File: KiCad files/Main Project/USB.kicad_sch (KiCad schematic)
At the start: 4 parts, among them J2 USB_C_Receptacle_USB2.0

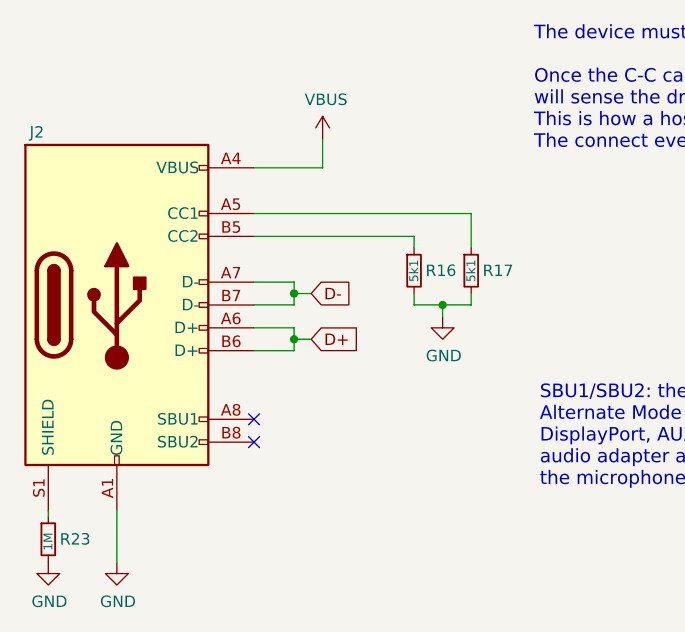
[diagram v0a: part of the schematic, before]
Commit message: shematic update
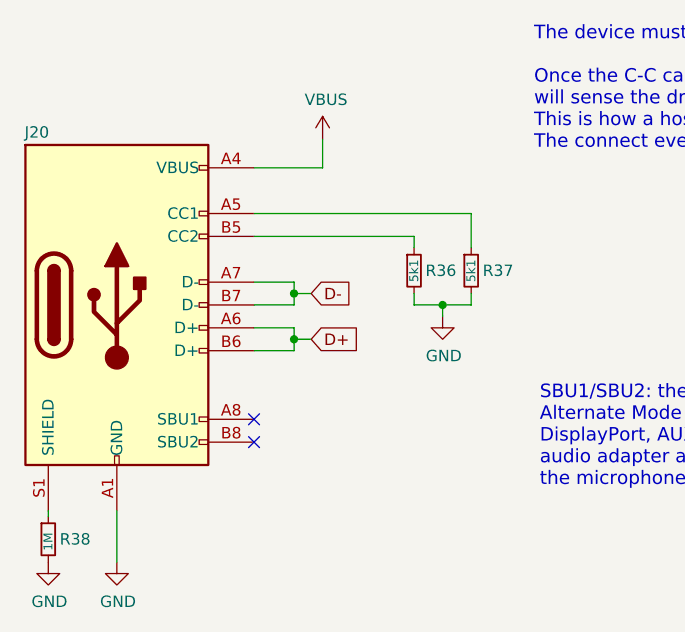
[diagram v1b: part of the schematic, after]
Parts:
- renumbered J2 to J20, R16 to R36, R17 to R37, R23 to R38
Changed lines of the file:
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@@
   (symbol (lib_id "Connector:USB_C_Receptacle_USB2.0") (at 96.52 94.615 0) (unit 1)
     (in_bom yes) (on_board yes)
-    (property "Reference" "J2" (id 0) (at 87.63 75.438 0))
+    (property "Reference" "J20" (id 0) (at 87.63 75.438 0))
     (property "Value" "USB_C_Receptacle_USB2.0" (id 1) (at 99.2378 74.9046 0)
       (effects (font (size 1.27 1.27)) hide)
@@
   (symbol (lib_id "power:VBUS") (at 119.38 76.2 0) (unit 1)
     (in_bom yes) (on_board yes)
-    (property "Reference" "#PWR070" (id 0) (at 119.38 80.01 0)
+    (property "Reference" "#PWR077" (id 0) (at 119.38 80.01 0)
       (effects (font (size 1.27 1.27)) hide)
     )
@@
   (symbol (lib_id "power:GND") (at 96.52 123.19 0) (unit 1)
     (in_bom yes) (on_board yes)
-    (property "Reference" "#PWR069" (id 0) (at 96.52 129.54 0)
+    (property "Reference" "#PWR080" (id 0) (at 96.52 129.54 0)
       (effects (font (size 1.27 1.27)) hide)
     )
@@
   (symbol (lib_id "Device:R_Small") (at 129.54 90.805 0) (unit 1)
     (in_bom yes) (on_board yes)
-    (property "Reference" "R16" (id 0) (at 130.81 90.805 0)
+    (property "Reference" "R36" (id 0) (at 130.81 90.805 0)
       (effects (font (size 1.27 1.27)) (justify left))
     )
@@
   (symbol (lib_id "Device:R_Small") (at 135.89 90.805 0) (unit 1)
     (in_bom yes) (on_board yes)
-    (property "Reference" "R17" (id 0) (at 137.16 90.805 0)
+    (property "Reference" "R37" (id 0) (at 137.16 90.805 0)
       (effects (font (size 1.27 1.27)) (justify left))
     )
@@
   (symbol (lib_id "power:GND") (at 132.715 95.885 0) (unit 1)
     (in_bom yes) (on_board yes)
-    (property "Reference" "#PWR072" (id 0) (at 132.715 102.235 0)
+    (property "Reference" "#PWR078" (id 0) (at 132.715 102.235 0)
       (effects (font (size 1.27 1.27)) hide)
     )
@@
   (symbol (lib_id "Device:R_Small") (at 88.9 120.65 0) (unit 1)
     (in_bom yes) (on_board yes)
-    (property "Reference" "R23" (id 0) (at 90.17 120.65 0)
+    (property "Reference" "R38" (id 0) (at 90.17 120.65 0)
       (effects (font (size 1.27 1.27)) (justify left))
     )
@@
   (symbol (lib_id "power:GND") (at 88.9 123.19 0) (unit 1)
     (in_bom yes) (on_board yes)
-    (property "Reference" "#PWR0272" (id 0) (at 88.9 129.54 0)
+    (property "Reference" "#PWR079" (id 0) (at 88.9 129.54 0)
       (effects (font (size 1.27 1.27)) hide)
     )

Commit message: update
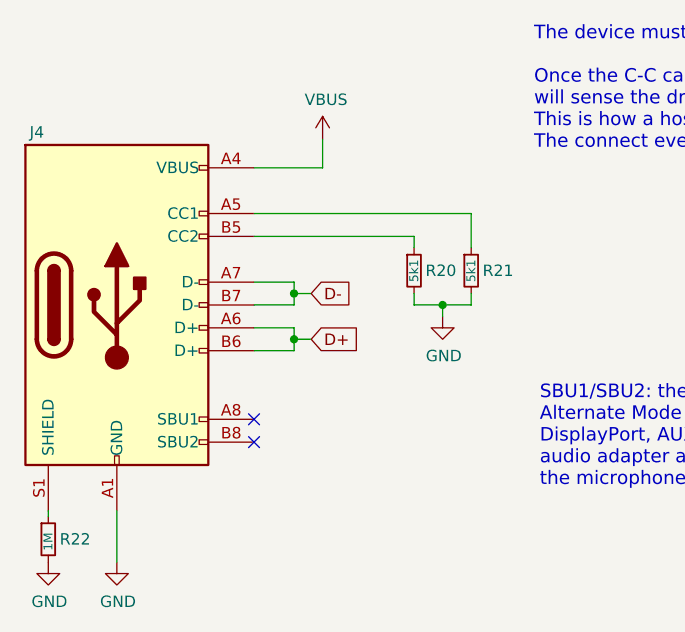
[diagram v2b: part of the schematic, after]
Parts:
- renumbered J20 to J4, R36 to R20, R37 to R21, R38 to R22
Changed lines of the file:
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@@
   (symbol (lib_id "Connector:USB_C_Receptacle_USB2.0") (at 96.52 94.615 0) (unit 1)
     (in_bom yes) (on_board yes)
-    (property "Reference" "J20" (id 0) (at 87.63 75.438 0))
+    (property "Reference" "J4" (id 0) (at 87.63 75.438 0))
     (property "Value" "USB_C_Receptacle_USB2.0" (id 1) (at 99.2378 74.9046 0)
       (effects (font (size 1.27 1.27)) hide)
@@
   (symbol (lib_id "power:VBUS") (at 119.38 76.2 0) (unit 1)
     (in_bom yes) (on_board yes)
-    (property "Reference" "#PWR077" (id 0) (at 119.38 80.01 0)
+    (property "Reference" "#PWR061" (id 0) (at 119.38 80.01 0)
       (effects (font (size 1.27 1.27)) hide)
     )
@@
   (symbol (lib_id "power:GND") (at 96.52 123.19 0) (unit 1)
     (in_bom yes) (on_board yes)
-    (property "Reference" "#PWR080" (id 0) (at 96.52 129.54 0)
+    (property "Reference" "#PWR064" (id 0) (at 96.52 129.54 0)
       (effects (font (size 1.27 1.27)) hide)
     )
@@
   (symbol (lib_id "Device:R_Small") (at 129.54 90.805 0) (unit 1)
     (in_bom yes) (on_board yes)
-    (property "Reference" "R36" (id 0) (at 130.81 90.805 0)
+    (property "Reference" "R20" (id 0) (at 130.81 90.805 0)
       (effects (font (size 1.27 1.27)) (justify left))
     )
@@
   (symbol (lib_id "Device:R_Small") (at 135.89 90.805 0) (unit 1)
     (in_bom yes) (on_board yes)
-    (property "Reference" "R37" (id 0) (at 137.16 90.805 0)
+    (property "Reference" "R21" (id 0) (at 137.16 90.805 0)
       (effects (font (size 1.27 1.27)) (justify left))
     )
@@
   (symbol (lib_id "power:GND") (at 132.715 95.885 0) (unit 1)
     (in_bom yes) (on_board yes)
-    (property "Reference" "#PWR078" (id 0) (at 132.715 102.235 0)
+    (property "Reference" "#PWR062" (id 0) (at 132.715 102.235 0)
       (effects (font (size 1.27 1.27)) hide)
     )
@@
   (symbol (lib_id "Device:R_Small") (at 88.9 120.65 0) (unit 1)
     (in_bom yes) (on_board yes)
-    (property "Reference" "R38" (id 0) (at 90.17 120.65 0)
+    (property "Reference" "R22" (id 0) (at 90.17 120.65 0)
       (effects (font (size 1.27 1.27)) (justify left))
     )
@@
   (symbol (lib_id "power:GND") (at 88.9 123.19 0) (unit 1)
     (in_bom yes) (on_board yes)
-    (property "Reference" "#PWR079" (id 0) (at 88.9 129.54 0)
+    (property "Reference" "#PWR063" (id 0) (at 88.9 129.54 0)
       (effects (font (size 1.27 1.27)) hide)
     )

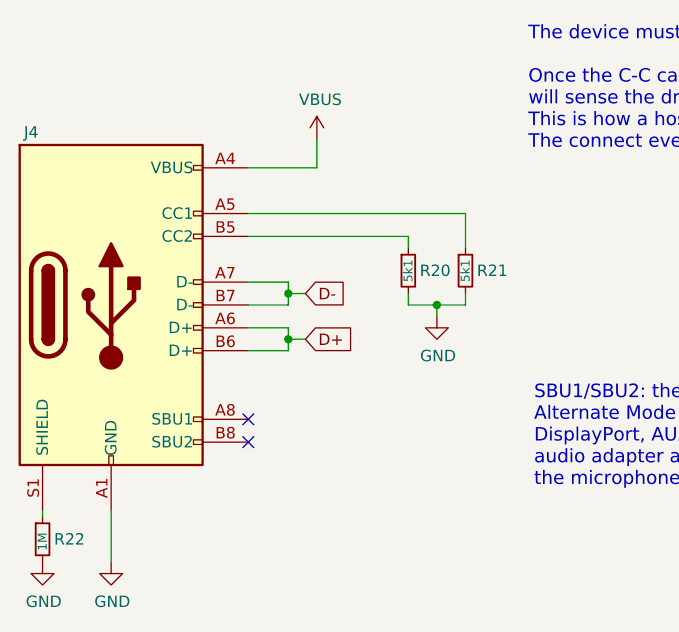
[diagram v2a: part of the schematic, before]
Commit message: update
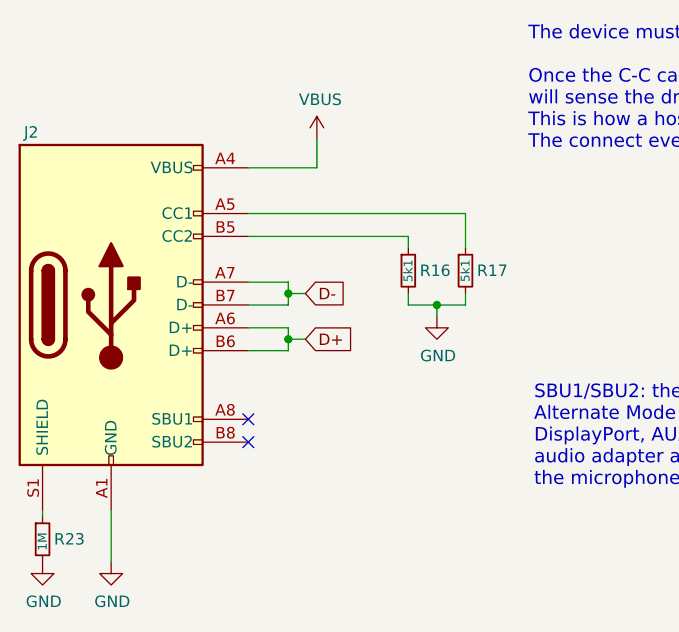
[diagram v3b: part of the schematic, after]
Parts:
- renumbered J4 to J2, R20 to R16, R21 to R17, R22 to R23
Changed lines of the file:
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@@
   (symbol (lib_id "Connector:USB_C_Receptacle_USB2.0") (at 96.52 94.615 0) (unit 1)
     (in_bom yes) (on_board yes)
-    (property "Reference" "J4" (id 0) (at 87.63 75.438 0))
+    (property "Reference" "J2" (id 0) (at 87.63 75.438 0))
     (property "Value" "USB_C_Receptacle_USB2.0" (id 1) (at 99.2378 74.9046 0)
       (effects (font (size 1.27 1.27)) hide)
@@
   (symbol (lib_id "power:VBUS") (at 119.38 76.2 0) (unit 1)
     (in_bom yes) (on_board yes)
-    (property "Reference" "#PWR061" (id 0) (at 119.38 80.01 0)
+    (property "Reference" "#PWR070" (id 0) (at 119.38 80.01 0)
       (effects (font (size 1.27 1.27)) hide)
     )
@@
   (symbol (lib_id "power:GND") (at 96.52 123.19 0) (unit 1)
     (in_bom yes) (on_board yes)
-    (property "Reference" "#PWR064" (id 0) (at 96.52 129.54 0)
+    (property "Reference" "#PWR069" (id 0) (at 96.52 129.54 0)
       (effects (font (size 1.27 1.27)) hide)
     )
@@
   (symbol (lib_id "Device:R_Small") (at 129.54 90.805 0) (unit 1)
     (in_bom yes) (on_board yes)
-    (property "Reference" "R20" (id 0) (at 130.81 90.805 0)
+    (property "Reference" "R16" (id 0) (at 130.81 90.805 0)
       (effects (font (size 1.27 1.27)) (justify left))
     )
@@
   (symbol (lib_id "Device:R_Small") (at 135.89 90.805 0) (unit 1)
     (in_bom yes) (on_board yes)
-    (property "Reference" "R21" (id 0) (at 137.16 90.805 0)
+    (property "Reference" "R17" (id 0) (at 137.16 90.805 0)
       (effects (font (size 1.27 1.27)) (justify left))
     )
@@
   (symbol (lib_id "power:GND") (at 132.715 95.885 0) (unit 1)
     (in_bom yes) (on_board yes)
-    (property "Reference" "#PWR062" (id 0) (at 132.715 102.235 0)
+    (property "Reference" "#PWR072" (id 0) (at 132.715 102.235 0)
       (effects (font (size 1.27 1.27)) hide)
     )
@@
   (symbol (lib_id "Device:R_Small") (at 88.9 120.65 0) (unit 1)
     (in_bom yes) (on_board yes)
-    (property "Reference" "R22" (id 0) (at 90.17 120.65 0)
+    (property "Reference" "R23" (id 0) (at 90.17 120.65 0)
       (effects (font (size 1.27 1.27)) (justify left))
     )
@@
   (symbol (lib_id "power:GND") (at 88.9 123.19 0) (unit 1)
     (in_bom yes) (on_board yes)
-    (property "Reference" "#PWR063" (id 0) (at 88.9 129.54 0)
+    (property "Reference" "#PWR0272" (id 0) (at 88.9 129.54 0)
       (effects (font (size 1.27 1.27)) hide)
     )
